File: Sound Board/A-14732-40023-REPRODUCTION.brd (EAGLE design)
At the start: 160.6 x 134 mm, 220 parts, among them P6 POWER, P7 SPEAKER, Q1 MPS3646, U1 OKI6295, U10 26LS32A, U11 26LS31, U12 27C040-150, U13 27C040-150, U14 YAMAHA 2151, U15 TIL7524, U16 74LS374, U17 74LS174, U18 16L8, U19 74LS11, U2 2064, U20 74LS139, U21 74LS14, U22 74LS74, U23 74LS74, U24 26LS31, U25 26LS32A, U26 74LS04, U28 YAMAHA 3012, U29 LM324D, U3 27C040, U30 MC3340, U31 MB3731, U32 TL084D, U33 TL084D, U4 6809E, U5 74LS374DW, U6 26LS32A, U7 26LS31, U8 74LS138, U9 74LS74, Y1 3.5749MHz, Y2 8MHz

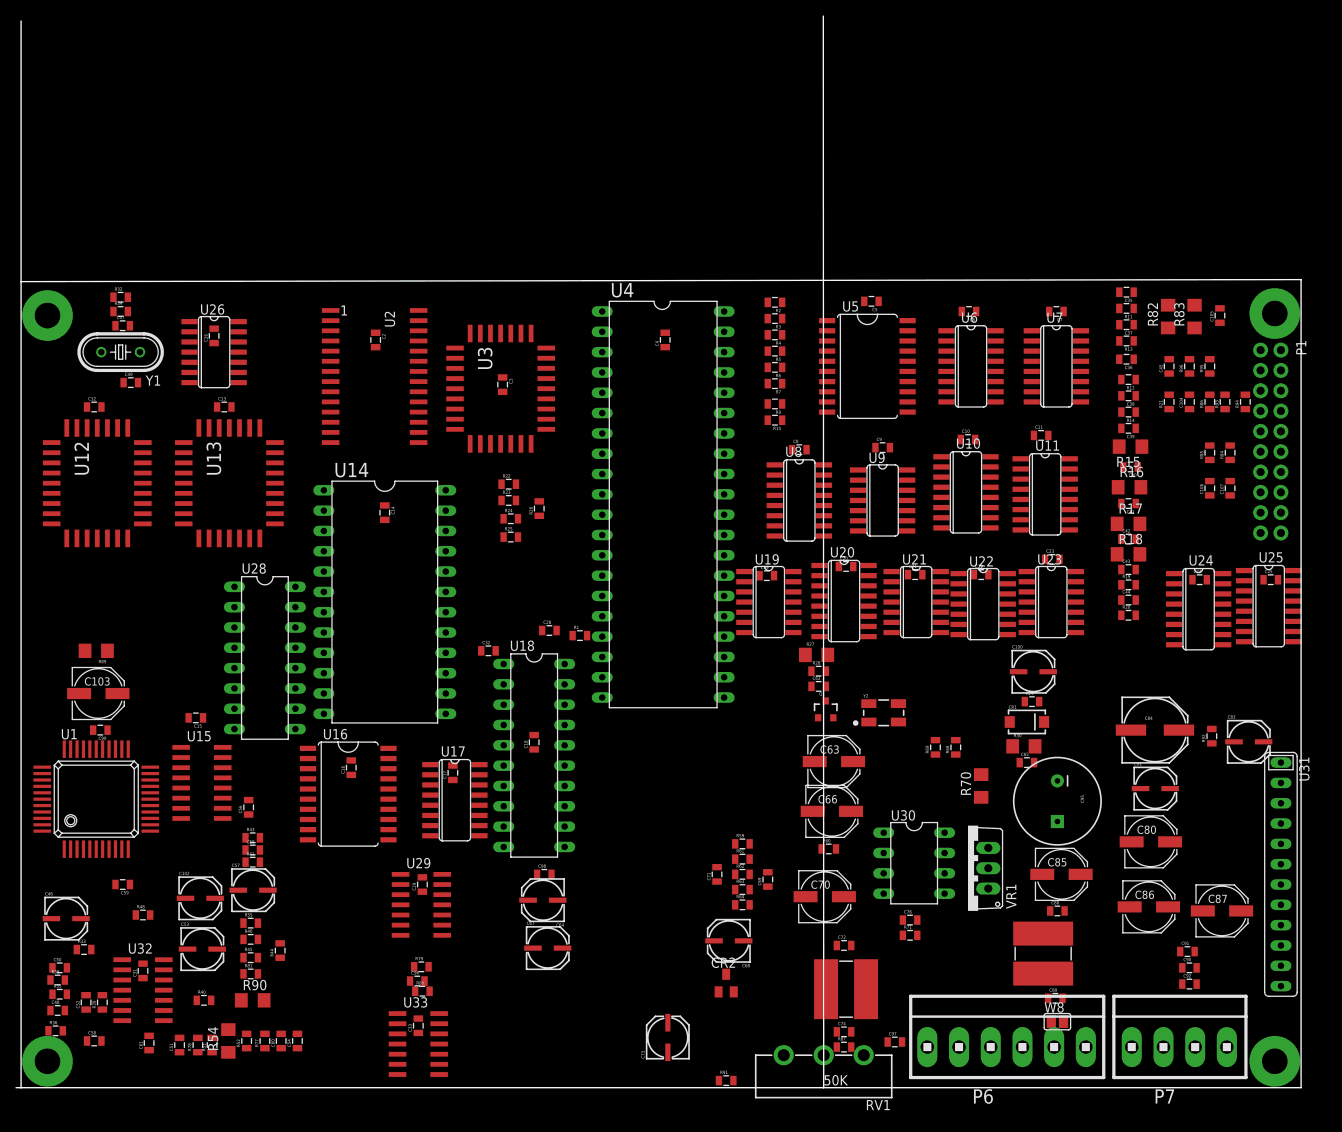
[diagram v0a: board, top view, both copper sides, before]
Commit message: board layout wip
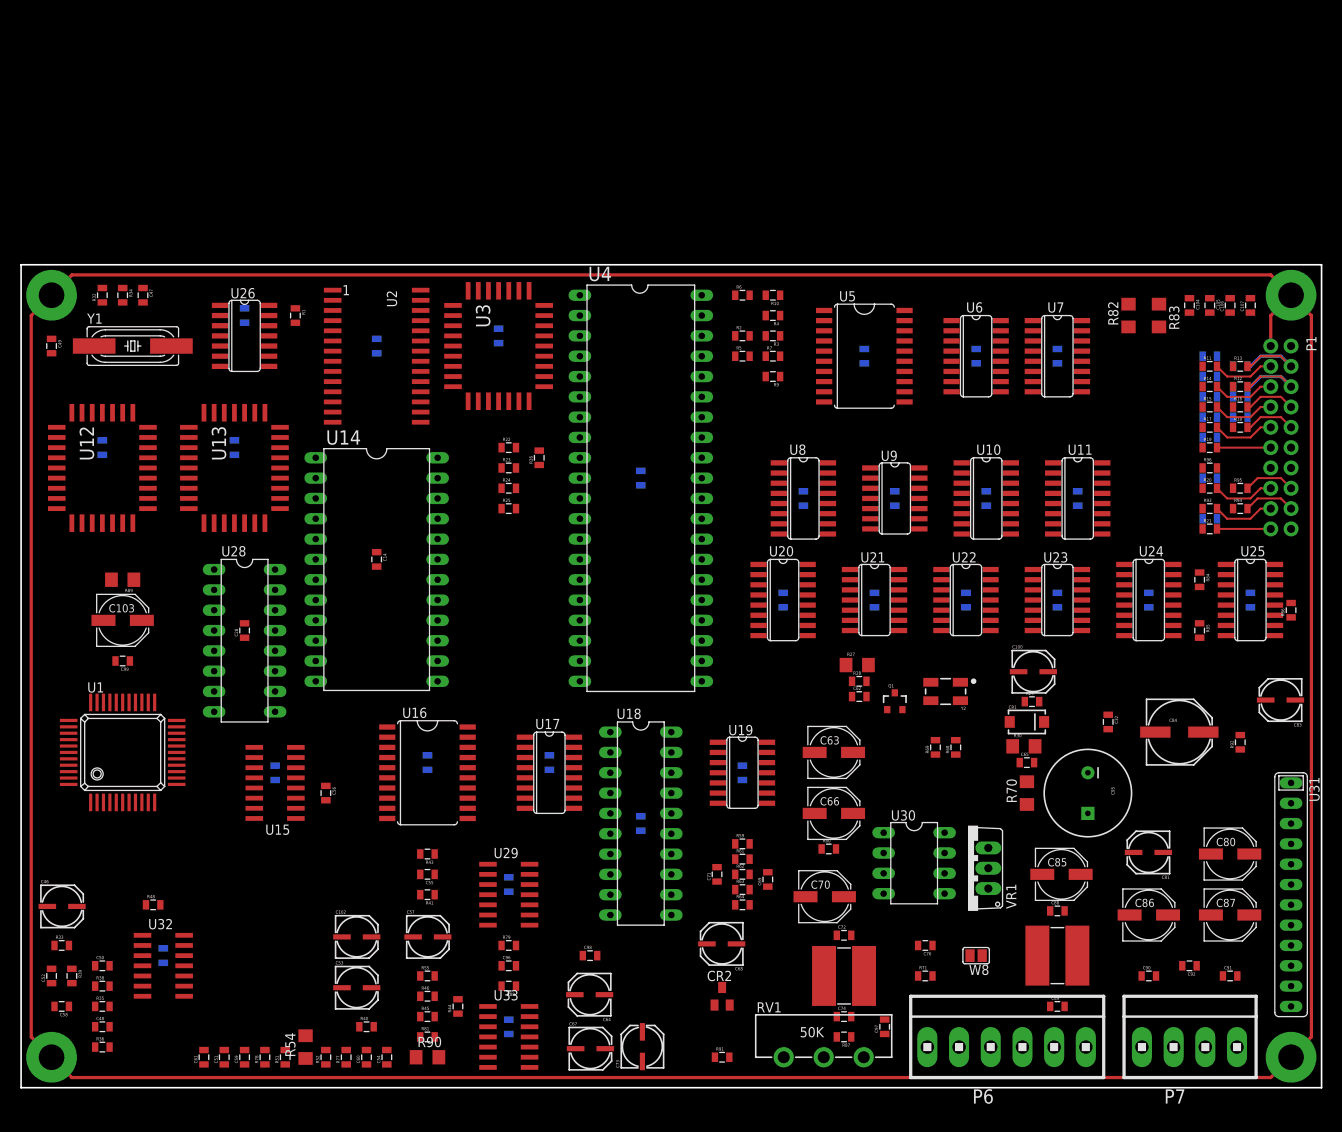
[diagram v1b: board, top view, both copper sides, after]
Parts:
- R15, R16, R17, R18: device resistor:R1206 -> SparkFun-Passives:0805
- Y1: device crystal:HC49U-V -> crystal:HC49UP
- moved C32 78.0 mm to (135.9, 45.7), turned to 270 degrees
- moved R1 53.5 mm to (34.3, 96.5), turned to 270 degrees
- moved C28 38.1 mm to (27.9, 57.1), turned to 90 degrees
- moved R86 27.9 mm to (158.8, 59.7)
- moved C59 26.4 mm to (27.9, 3.81), turned to 90 degrees
- moved C19 24.8 mm to (90.2, 39.4), flipped to the bottom, turned to 90 degrees
- moved R81 23.5 mm to (50.8, 6.35)
- moved R44 23.3 mm to (54.6, 10.2)
- moved R45 23.3 mm to (50.8, 8.89)
- moved R46 23.2 mm to (50.8, 11.4)
- moved R55 23.1 mm to (50.8, 14.0)
- moved C106 23.0 mm to (151.1, 97.8)
- moved C107 23.0 mm to (153.7, 97.8)
- moved R90 23.0 mm to (50.8, 3.81)
- moved C57 22.6 mm to (50.8, 19.1)
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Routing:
- net GND: track 0.00 -> 516.2 mm
- net SND_DAT3: track 0.00 -> 13.0 mm
- net SND_DAT1: track 0.00 -> 13.0 mm
- net SND_DAT4: track 0.00 -> 7.77 mm
- net B_SND_RD: track 0.00 -> 7.77 mm
- net SND_DAT6: track 0.00 -> 7.77 mm
- net SND_DAT2: track 0.00 -> 7.77 mm
- net SND_DAT0: track 0.00 -> 7.77 mm
- net N$101: track 0.00 -> 7.77 mm
- net SND_RDY: track 0.00 -> 6.72 mm
- net SND_DAV: track 0.00 -> 6.72 mm
- net N$99: track 0.00 -> 6.50 mm
- net N$102: track 0.00 -> 6.50 mm
- net SND_DAT7: track 0.00 -> 6.50 mm
- net SND_DAT5: track 0.00 -> 6.50 mm
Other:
- board size 160.6 x 134 mm -> 162.6 x 102.9 mm
